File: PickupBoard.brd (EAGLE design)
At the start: 47.9 x 29 mm, 22 parts, among them IC2 TL072

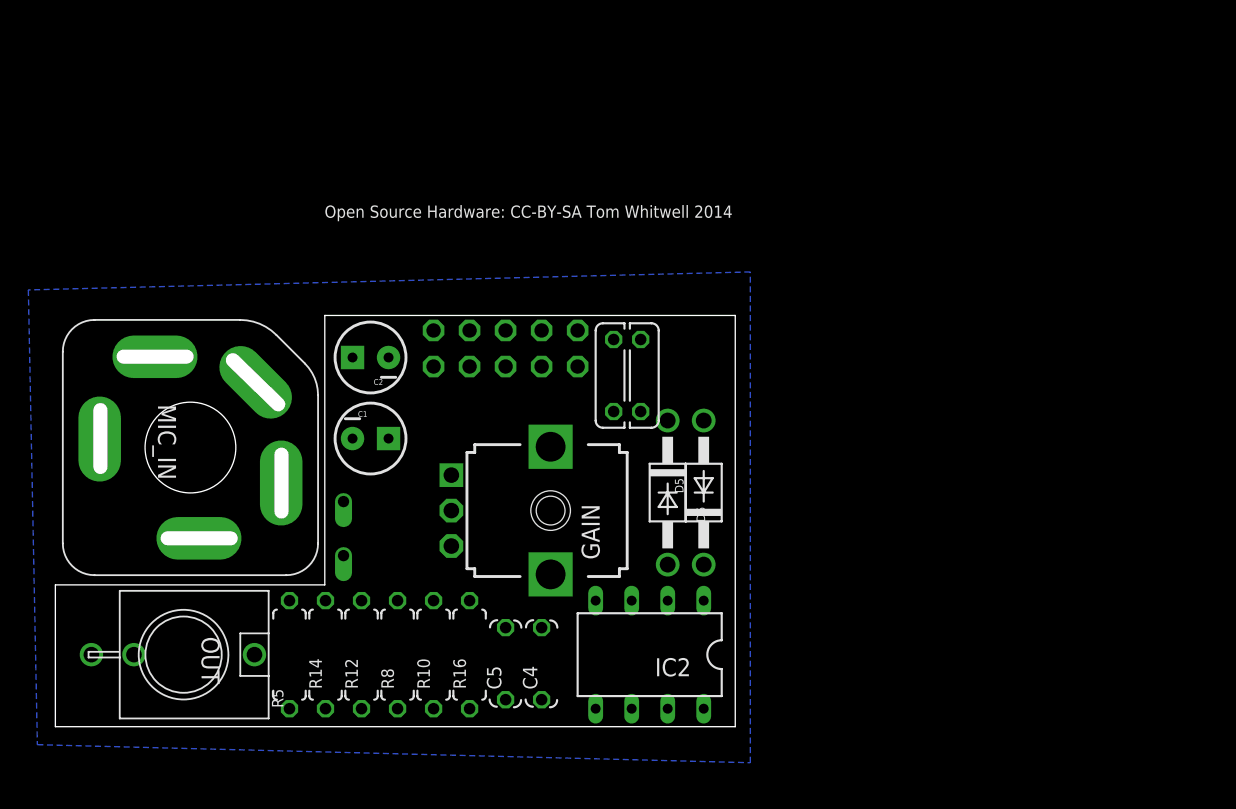
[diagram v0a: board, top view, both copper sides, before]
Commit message: Building the circuit
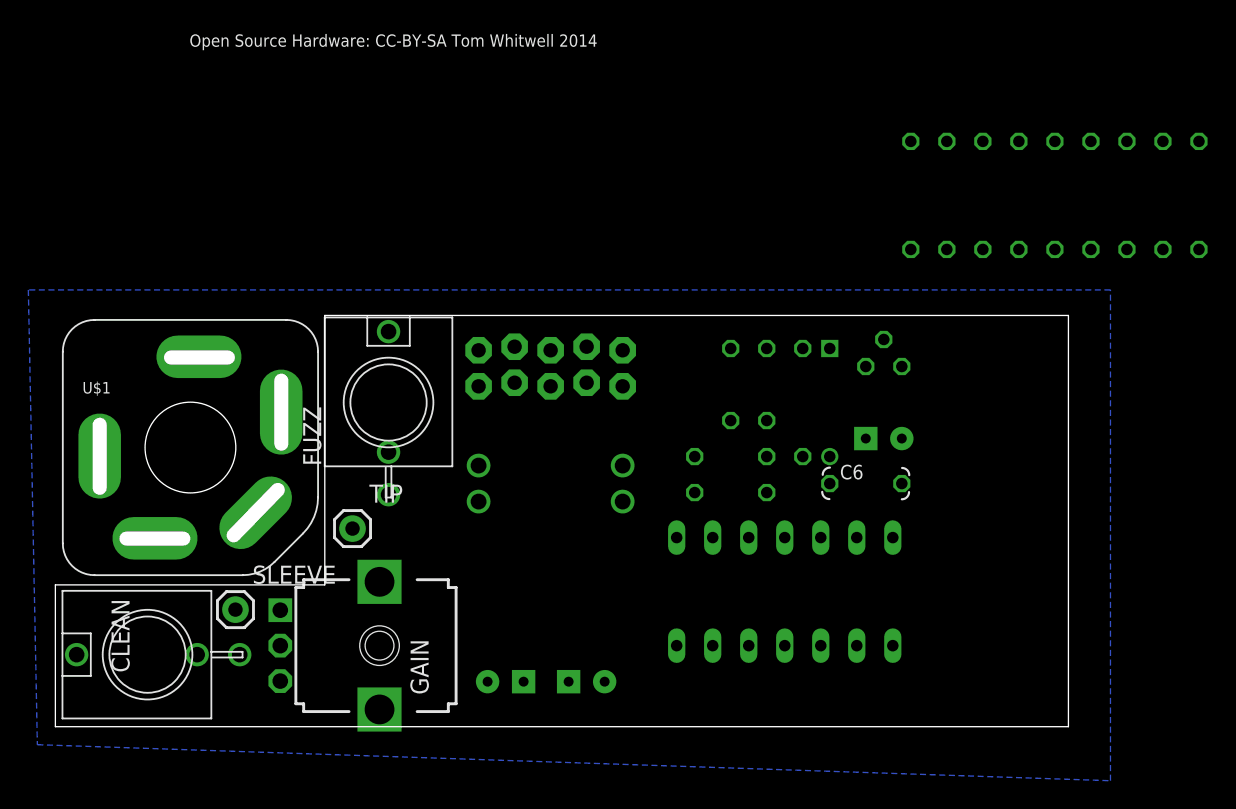
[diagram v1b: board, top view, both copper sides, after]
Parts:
- removed IC2: TL072, TomW:DIL08
- removed OUT: THONKICONNNEW, MusicThingModular:WQP-PJ301M-12_JACK
- removed PICKUP: MIC+, TomW:LONG_PAD_1
- removed PICKUP_GND: MIC-, TomW:LONG_PAD_1
- removed SV1: (no value), TomW:MA05-2
- added 4148: (no value), MusicThingModular:DO35-7
- added C3: 4.7f, SparkFun-Passives:CPOL-RADIAL-10UF-25V
- added C6: 100n, TomW:C050-024X044
- added CLEAN, FUZZ: THONKICONNNEW, MusicThingModular:WQP-PJ301M-12_JACK
- added R1: 100k, MusicThingModular:7MM_RESISTOR
- added R2: 220R, MusicThingModular:7MM_RESISTOR
- added R3: 2.2k, MusicThingModular:7MM_RESISTOR
- added R4: 22k, MusicThingModular:7MM_RESISTOR
- added SLEEVE, TIP: M01PTH, SparkFun-Connectors:1X01
- added T1: 2N3904, transistor:TO92
- added U1: TL074_, MusicThingModular:DIL14
- U$2: value (none) -> EURO_POWER_LOCK; device TW_logos:MTM_2CM_SCREEN_200DPI -> MusicThingModular:EURO_PWR_HEADER_LOCK
- moved R5 71.8 mm to (80.6, 37.5), flipped to the bottom
- moved R10 54.5 mm to (70.5, 37.5), flipped to the bottom
- moved R12 54.5 mm to (65.4, 37.5), flipped to the bottom
- moved R14 54.5 mm to (62.9, 37.5), flipped to the bottom
- moved R8 54.5 mm to (67.9, 37.5), flipped to the bottom
- moved R16 44.9 mm to (60.3, 37.5), flipped to the bottom
- moved U$2 38.1 mm to (34.9, 25.4), turned to 180 degrees
- moved C2 24.8 mm to (31.8, 3.17), flipped to the bottom
- moved C1 22.9 mm to (37.5, 3.17), flipped to the bottom
- moved C5 19.9 mm to (47.6, 16.5), flipped to the bottom, turned to 180 degrees
- moved C4 19.8 mm to (47.6, 19.1), flipped to the bottom, turned to 180 degrees
- moved GAIN 15.4 mm to (22.9, 5.71)
- moved D6 11.0 mm to (34.9, 18.4), flipped to the bottom, turned to 0 degrees
- moved FUSE 8.91 mm to (50.2, 24.1), flipped to the bottom, turned to 90 degrees
- moved 1 8.28 mm to (47.6, 24.1), flipped to the bottom
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- renumbered MIC_IN to U$1
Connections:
- new net FUZZ_IN: C3.1
- new net N$11: R3.2, R4.2, U1.13
- new net N$12: R2.1, R4.1, U1.14
- new net N$13: FUZZ.P$1_TIP, R2.2
- new net N$7: 4148.C, C3.2, T1.2
- new net N$9: 4148.A, C6.1, R1.1, T1.1
- net +12V: now also R1.2, U1.4; no longer IC2.8
- net +12V_INLET: now also U$2.POS1, U$2.POS2; no longer SV1.10, SV1.9
- net -12V: now also U1.11; no longer IC2.4
- net -12V_INLET: now also U$2.NEG1, U$2.NEG2; no longer SV1.1, SV1.2
- net GND: now also CLEAN.P$3_SLEEVE, FUZZ.P$3_SLEEVE, R3.1, SLEEVE.1, T1.3, U$2.GND1, U$2.GND2, U$2.GND3, U$2.GND4, U$2.GND5, U$2.GND6; no longer OUT.P$3_SLEEVE, PICKUP_GND.P$1, SV1.3, SV1.4, SV1.5, SV1.6, SV1.7, SV1.8, U$1.SLEEVE
- net N$1: now also C6.2, U1.12; no longer PICKUP.P$1, U$1.TIP_SW
- net N$10: now also CLEAN.P$1_TIP; no longer OUT.P$1_TIP
- net N$2: now also TIP.1, U1.3; no longer IC2.3, U$1.TIP
- net N$3: now also U1.2; no longer IC2.2
- net N$4: now also U1.1, U1.5; no longer IC2.1, IC2.5
- net N$6: now also U1.6; no longer IC2.6
- net N$8: now also U1.7; no longer IC2.7
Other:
- board size 47.9 x 29 mm -> 71.4 x 29 mm
